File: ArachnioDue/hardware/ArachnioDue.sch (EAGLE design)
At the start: 68 parts, among them J5 HEAD17-NOSS, J6 HEAD17-NOSS, Q1 12MHz, U1 SAM3SA-MU, U2 AP2111HA-3.3, U5 ESP8266EX, U6 SPI_FLASH, Y1 26 MHz/10 pF

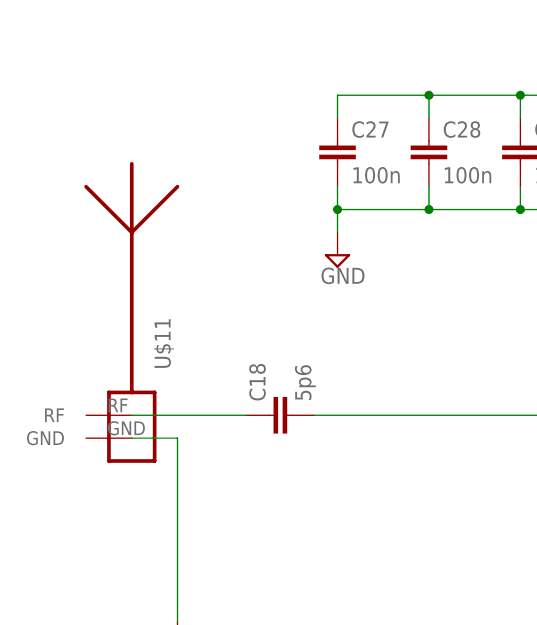
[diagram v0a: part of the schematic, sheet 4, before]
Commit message: Pre-prototype check-in
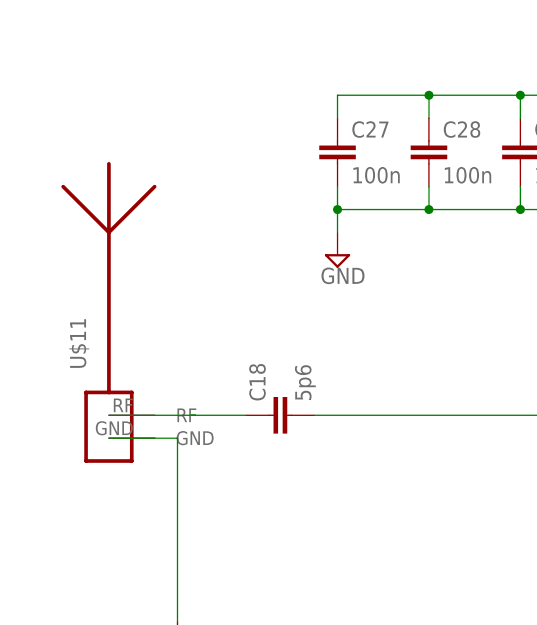
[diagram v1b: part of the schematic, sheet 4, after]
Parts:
- C1: PARTNO C0603C105K3PACTU -> generic MLCC:1u/25V/0603
- C10, C23, C24, C25, C26, C6, C7: PARTNO CL21F475ZPFNNNE -> generic MLCC:4u7/10V/0603
- C11, C13, C15, C20, C21, C22, C27, C28, C29, C5: PARTNO CC0402KRX7R7BB104 -> generic MLCC:100n/16V/0402
- C12, C2: PARTNO (none) -> generic MLCC:100n/16V/0402
- C14: PARTNO JMK107BJ225KAHT -> generic MLCC:2u2/6V3/0603
- C16, C17: PARTNO C0603C100K5GACTU -> (none)
- C18: PARTNO 251R14S5R6CV4T -> (none)
- C19: PARTNO CC0603ZRY5V9BB104 -> generic MLCC:100n/16V/0402
- C3, C4, C8: PARTNO CL10A475KA8NQNC -> generic MLCC:4u7/25V/0603
- C9: PARTNO CC0603ZRY5V9BB104 -> generic MLCC:100n/50V/0603
- CN1: PARTNO USB-M26FTR -> 10104111-0001LF
- D1, D2: PARTNO (none) -> CDBW140-G
- J5, J6, LOAD/OTA: BOM (none) -> EXCLUDE
- Q1: PARTNO (none) -> PRQC12.00CR1010V00L
- R1, R10, R11, R14, R2, R9: PARTNO RNCP0603FTD10K0 -> generic resistor:10K/0402
- R13: PARTNO MCR03ERTJ201 -> generic resistor:200R/0402
- R3: PARTNO RMCF0603FT12K0 -> generic resistor:12K/0402
- R5, R7, R8: PARTNO RMCF0603FT1K00 -> generic resistor:1K/0402
- RN1: PARTNO (none) -> EXB-V4V270JV
- U1: PARTNO (none) -> ATSAM4S2AA-MU
- Y2: PARTNO (none) -> MC-146 32.768KA-AC3
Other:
- moved on the sheet: U$11
